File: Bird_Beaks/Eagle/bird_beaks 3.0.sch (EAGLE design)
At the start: 29 parts, among them U1 ADAFRUIT_ITSYBITSY_5V, X1 PHOENIX_508_3PIN, X10 PHOENIX_508_3PIN, X11 PHOENIX_508_4PIN, X2 PHOENIX_508_3PIN, X3 PHOENIX_508_3PIN, X4 PHOENIX_508_2PIN, X5 PHOENIX_508_4PIN, X6 PHOENIX_508_4PIN, X7 PHOENIX_508_3PIN, X8 PHOENIX_508_3PIN, X9 PHOENIX_508_3PIN

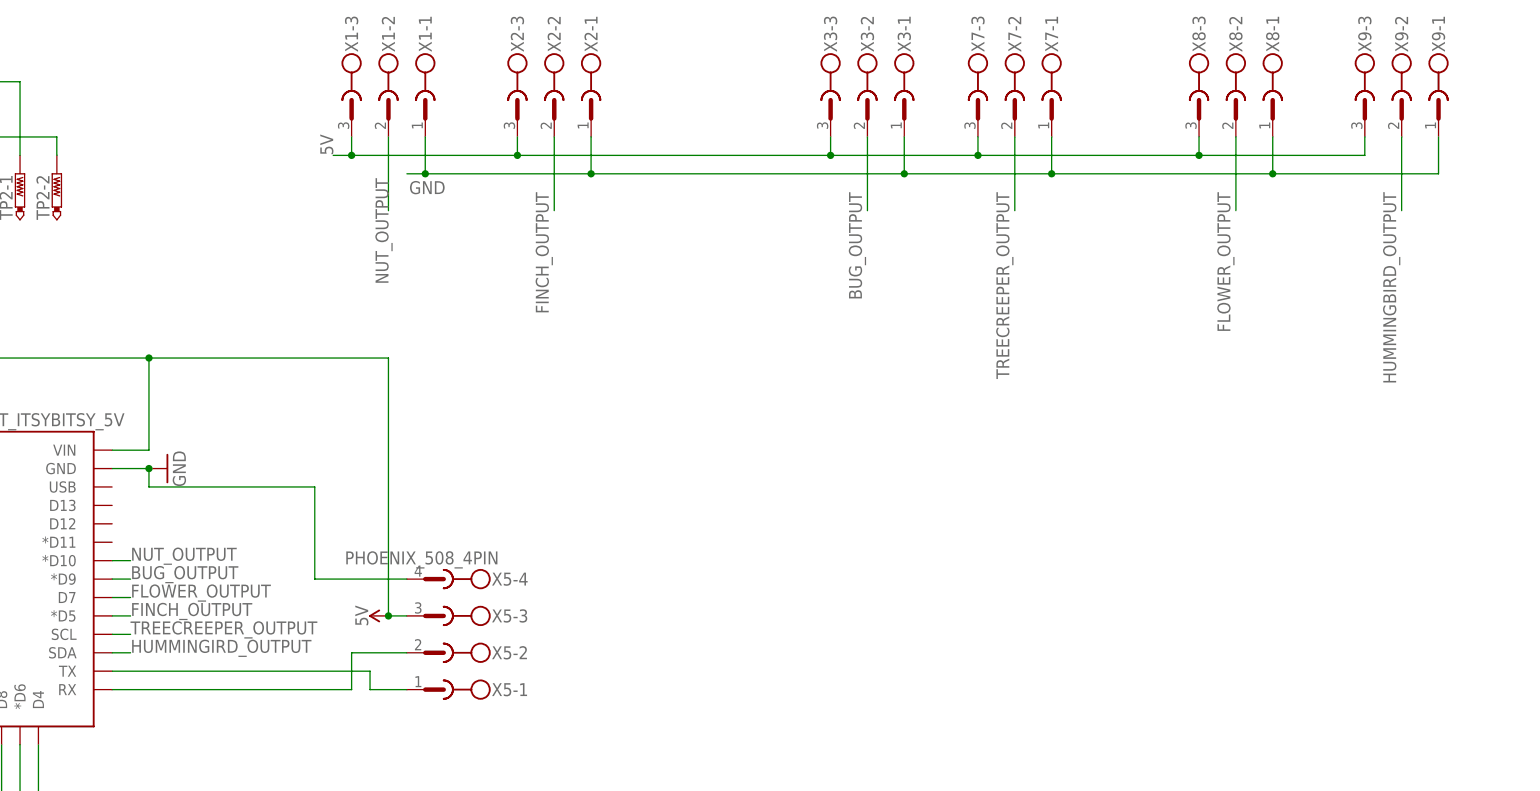
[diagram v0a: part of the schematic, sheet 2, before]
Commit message: Revision for output
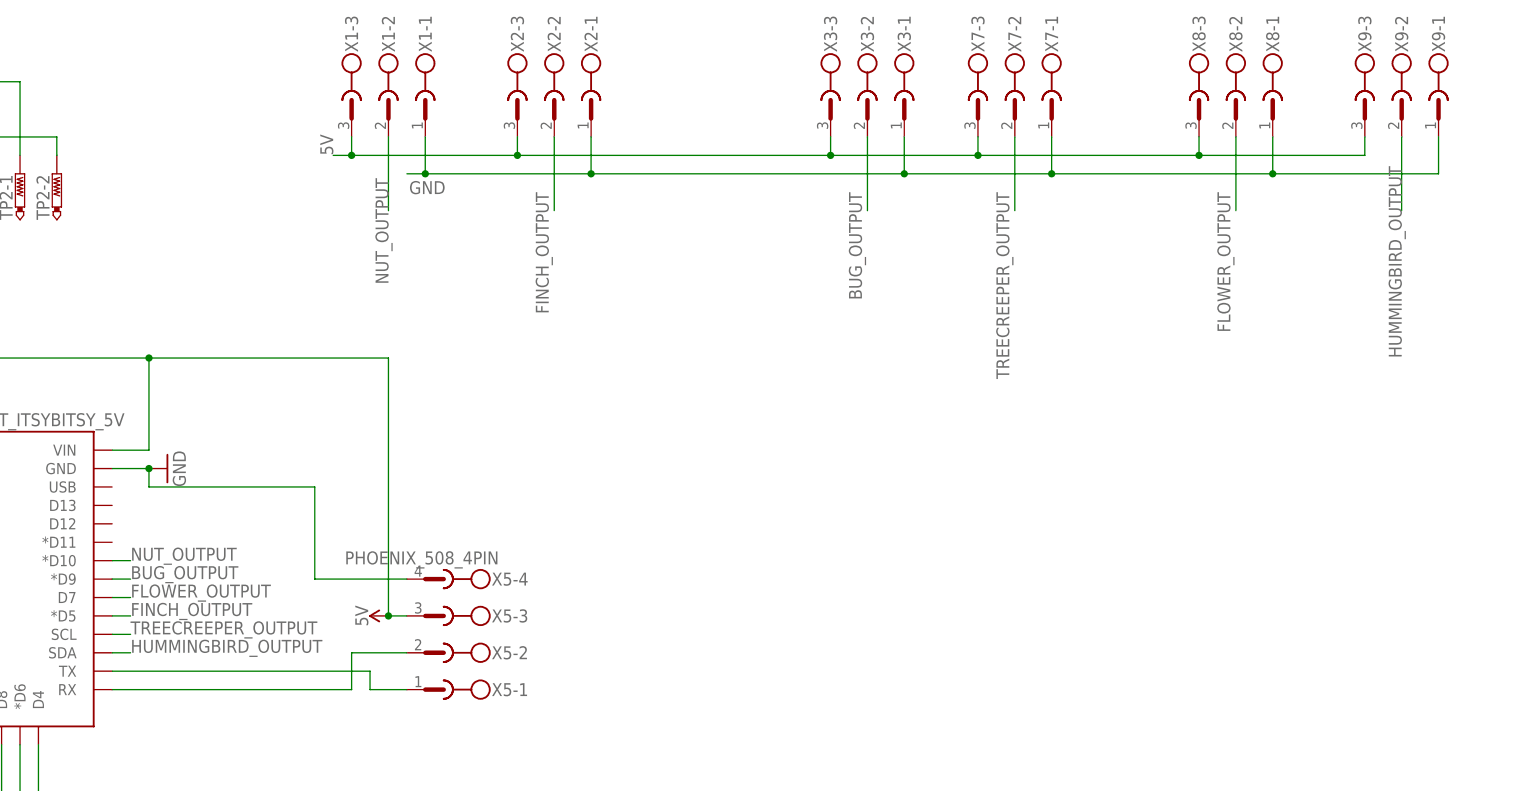
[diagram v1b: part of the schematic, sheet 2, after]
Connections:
- removed net HUMMINGIRD_OUTPUT: U1.SDA
- net HUMMINGBIRD_OUTPUT: now also U1.SDA
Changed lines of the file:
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@@
 <class number="0" name="Low Power" width="0.1524" drill="0.254">
 </class>
-<class number="1" name="High Power" width="0.762" drill="0.4826">
+<class number="1" name="High Power" width="1.27" drill="0.4826">
 </class>
 </classes>
@@
 </segment>
 </net>
-<net name="HUMMINGIRD_OUTPUT" class="0">
-<segment>
-<pinref part="U1" gate="G$1" pin="SDA"/>
-<wire x1="114.3" y1="134.62" x2="116.84" y2="134.62" width="0.1524" layer="91"/>
-<label x="116.84" y="134.62" size="1.778" layer="95"/>
-</segment>
-</net>
 <net name="TREECREEPER_OUTPUT" class="0">
 <segment>
@@
 </segment>
 </net>
-<net name="HUMMINGBIRD_OUTPUT" class="0">
-<segment>
-<pinref part="X9" gate="-2" pin="1"/>
-<wire x1="292.1" y1="205.74" x2="292.1" y2="195.58" width="0.1524" layer="91"/>
-<label x="289.56" y="198.12" size="1.778" layer="95" rot="R270"/>
-</segment>
-</net>
 <net name="12V" class="1">
 <segment>
@@
 </segment>
 </net>
+<net name="HUMMINGBIRD_OUTPUT" class="0">
+<segment>
+<pinref part="U1" gate="G$1" pin="SDA"/>
+<wire x1="114.3" y1="134.62" x2="116.84" y2="134.62" width="0.1524" layer="91"/>
+<label x="116.84" y="134.62" size="1.778" layer="95"/>
+</segment>
+<segment>
+<pinref part="X9" gate="-2" pin="1"/>
+<wire x1="292.1" y1="205.74" x2="292.1" y2="195.58" width="0.1524" layer="91"/>
+<label x="292.1" y="175.26" size="1.778" layer="95" rot="R90"/>
+</segment>
+</net>
